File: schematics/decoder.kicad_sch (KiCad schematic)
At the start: 3 parts, among them U23 ATF22V10C-7, U25 ATF22V10C-7, U26 74HC373

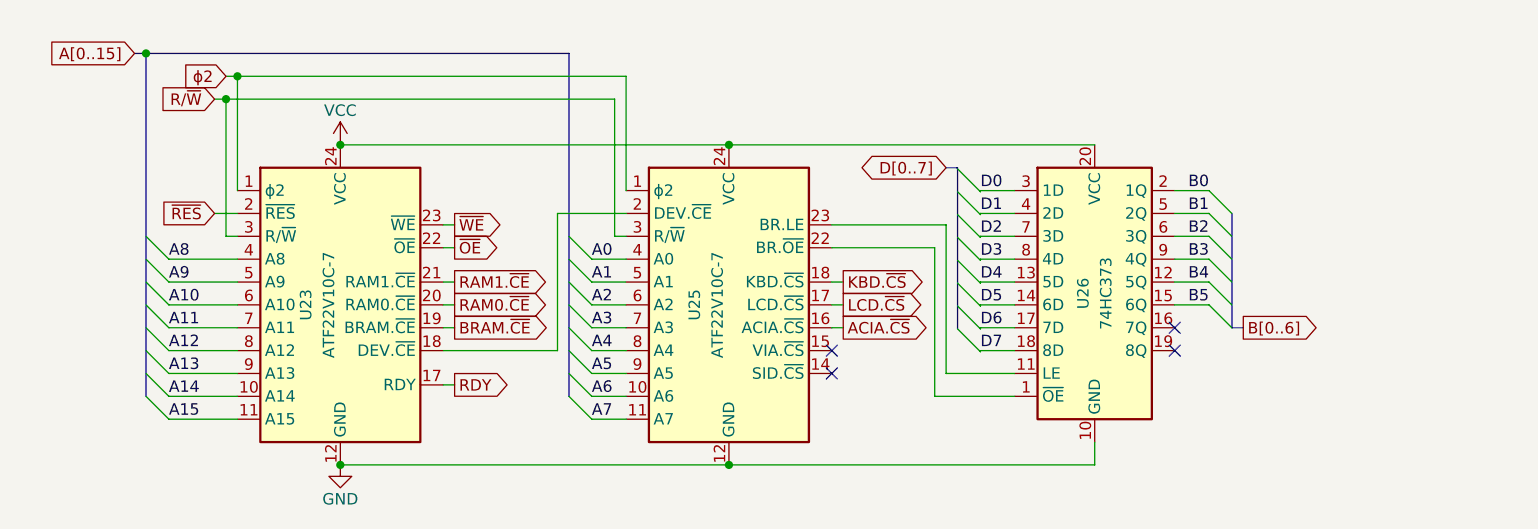
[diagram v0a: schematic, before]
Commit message: added phi0 for write latch timing
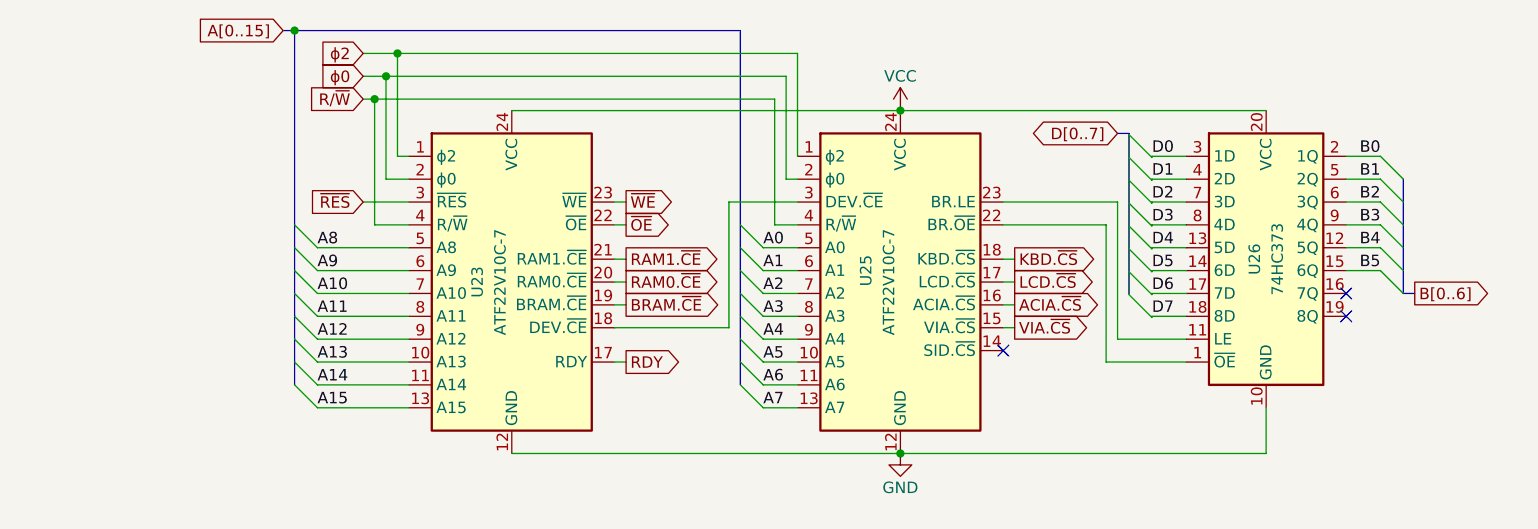
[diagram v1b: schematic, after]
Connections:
- net A0: now also U25.5 (A0); no longer U25.4 (A0)
- net A1: now also U25.6 (A1); no longer U25.5 (A1)
- net A10: now also U23.7 (A10); no longer U23.6 (A10)
- net A11: now also U23.8 (A11); no longer U23.7 (A11)
- net A12: now also U23.9 (A12); no longer U23.8 (A12)
- net A13: now also U23.10 (A13); no longer U23.9 (A13)
- net A14: now also U23.11 (A14); no longer U23.10 (A14)
- net A15: now also U23.13 (A15); no longer U23.11 (A15)
- net A2: now also U25.7 (A2); no longer U25.6 (A2)
- net A3: now also U25.8 (A3); no longer U25.7 (A3)
- net A4: now also U25.9 (A4); no longer U25.8 (A4)
- net A5: now also U25.10 (A5); no longer U25.9 (A5)
- net A6: now also U25.11 (A6); no longer U25.10 (A6)
- net A7: now also U25.13 (A7); no longer U25.11 (A7)
- net A8: now also U23.5 (A8); no longer U23.4 (A8)
- net A9: now also U23.6 (A9); no longer U23.5 (A9)
- net R/~{W}: now also U23.4 (R/~{W}), U25.4 (R/~{W}); no longer U23.3 (R/~{W}), U25.3 (R/~{W})
- net ~{RES}: now also U23.3 (~{RES}); no longer U23.2 (~{RES})
- net VIA.~{CS}: now reaches U25.15 (VIA.~{CS})
- net at U23.18 (DEV.~{CE}): now also U25.3 (DEV.~{CE}); no longer U25.2 (DEV.~{CE})
- new net ϕ0: U23.2 (ϕ0), U25.2 (ϕ0)
- no-connect marks 4 -> 3
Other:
- moved on the sheet: U26
